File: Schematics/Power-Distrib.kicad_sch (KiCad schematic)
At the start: 49 parts, among them J102 Jack-DC, J103 Conn_01x02, J18 Jack-DC, J24 Conn_01x02, J25 Conn_01x02, J26 Screw_Terminal_01x02, J27 Conn_01x02, J28 Conn_01x02, J29 Conn_01x02, J30 Conn_01x02, J31 Conn_01x02, J32 Conn_01x02, J33 Screw_Terminal_01x02, J34 Conn_01x03, J35 Conn_01x03, J36 Conn_01x03, J37 Conn_01x03, J38 Conn_01x03, J39 Conn_01x03, J40 Conn_01x03, J41 Conn_01x03, J42 Conn_01x03, J43 Screw_Terminal_01x02, K1 Relay_SPDT, U19 LM7805, U20 LM7805, U21 LM7812, U22 LM7912

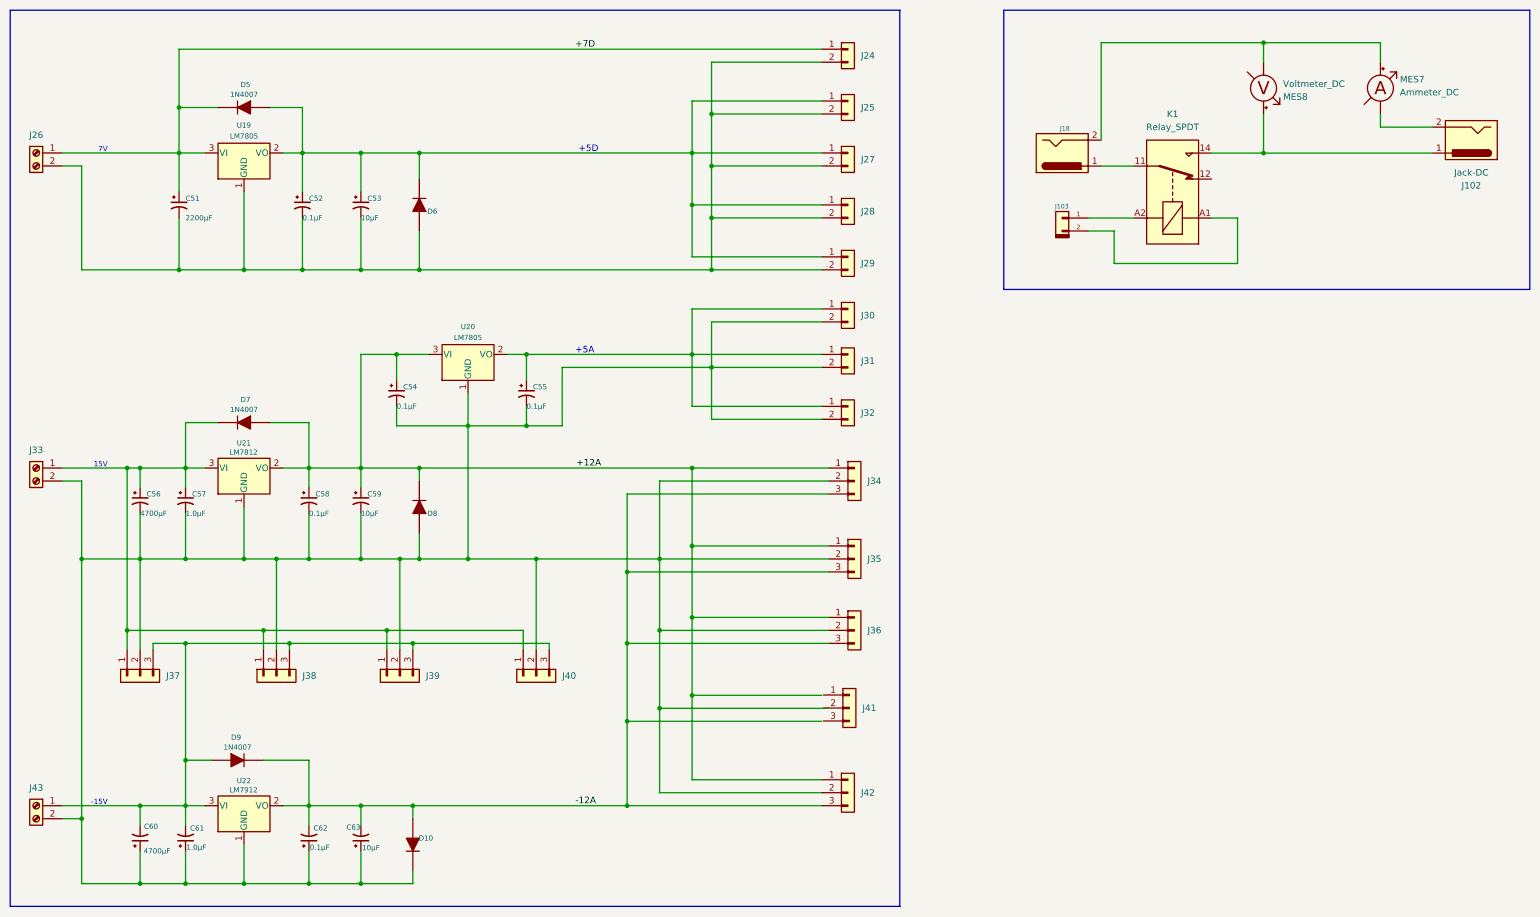
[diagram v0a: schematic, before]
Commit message: updated schematics.
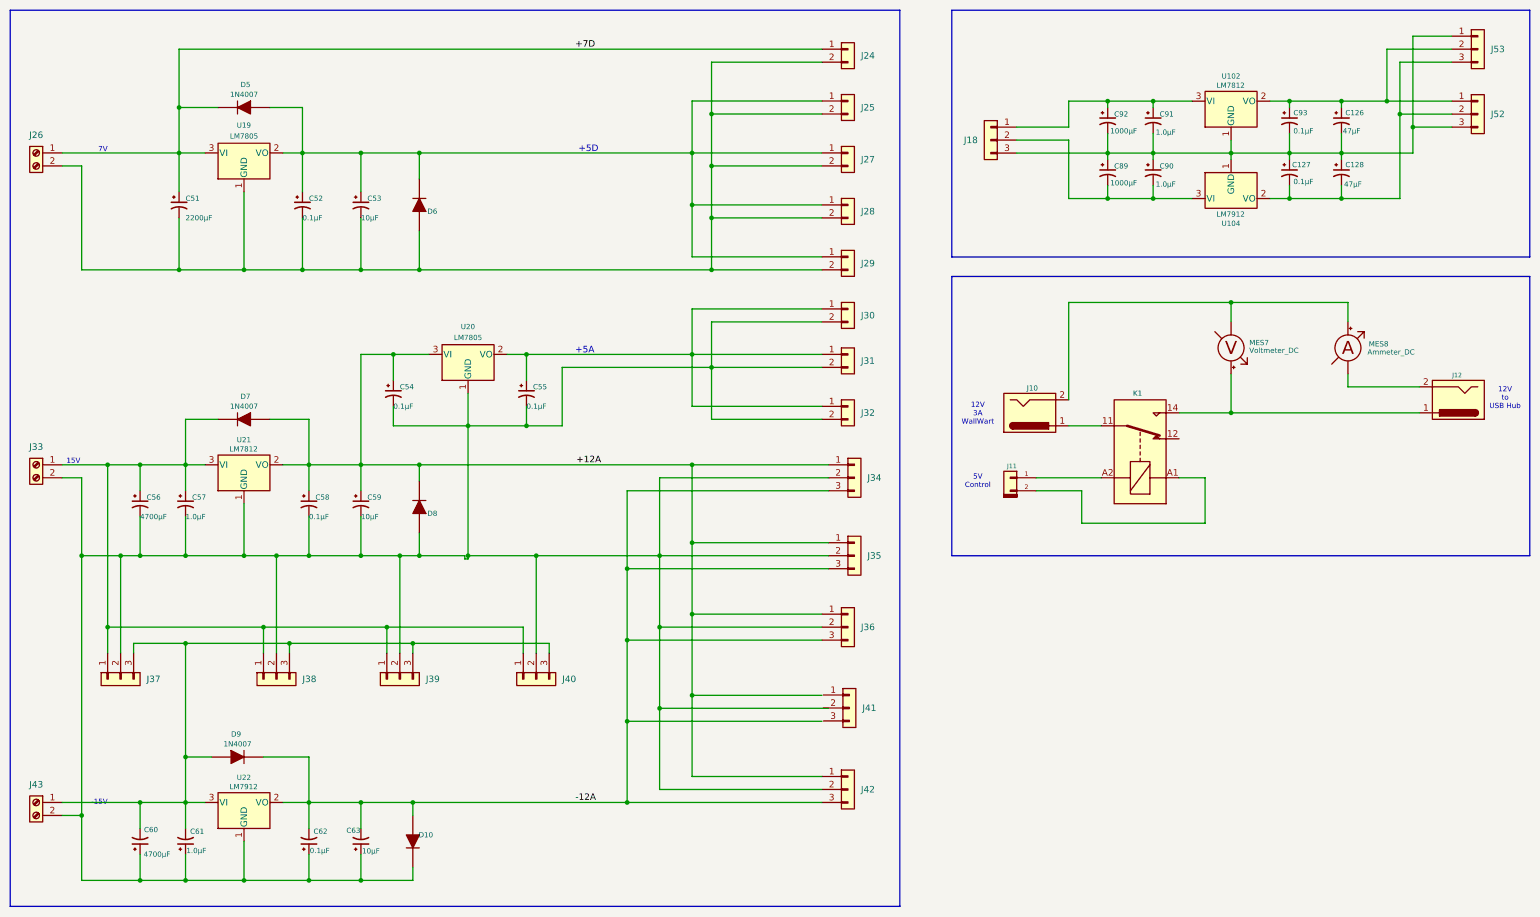
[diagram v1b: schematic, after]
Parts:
- removed J102, J18: Jack-DC, symbol Connector:Jack-DC
- removed J103: Conn_01x02, symbol My Connectors:Conn_01x02
- removed MES7: Ammeter_DC, symbol Device:Ammeter_DC
- removed MES8: Voltmeter_DC, symbol Device:Voltmeter_DC
- added C126, C128: 47µF, symbol Device:C_Polarized_Small_US
- added C127, C93: 0.1µF, symbol Device:C_Polarized_Small_US
- added C89, C92: 1000µF, symbol Device:C_Polarized_Small_US
- added C90, C91: 1.0µF, symbol Device:C_Polarized_Small_US
- added J10, J12: Jack-DC, symbol Connector:Jack-DC
- added J11: Conn_01x02, symbol My Connectors:Conn_01x02
- added J18, J52, J53: Conn_01x03, symbol Connector_Generic:Conn_01x03
- added MES7: Voltmeter_DC, symbol Device:Voltmeter_DC
- added MES8: Ammeter_DC, symbol Device:Ammeter_DC
- added U102: LM7812, symbol Regulator_Linear:LM1117-5.0
- added U104: LM7912, symbol Regulator_Linear:LM1117-5.0
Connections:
- net at K1.11: now also J10.1
- net at K1.14: now also J12.1, MES7.2 (+)
- net at K1.A2: now also J11.1 (Pin_1)
- net at K1.A1: now also J11.2 (Pin_2)
- new net: C126.2, C127.1, C128.1, C89.1, C90.1, C91.2, C92.2, C93.2, J18.3 (Pin_3), J52.3 (Pin_3), J53.1 (Pin_1), U102.1 (GND), U104.1 (GND)
- new net: C126.1, C93.1, J52.1 (Pin_1), J53.2 (Pin_2), U102.2 (VO)
- new net: C127.2, C128.2, J52.2 (Pin_2), J53.3 (Pin_3), U104.2 (VO)
- new net: C91.1, C92.1, J18.1 (Pin_1), U102.3 (VI)
- new net: C89.2, C90.2, J18.2 (Pin_2), U104.3 (VI)
- new net: J10.2, MES7.1 (-), MES8.2 (+)
- new net: J12.2, MES8.1 (-)
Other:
- note added: "12V 3A WallWart"
- note added: "12V to USB Hub"
- note added: "5V Control"
- moved on the sheet: C54, C56, C57, C58, C59, C60, C61, C62, C63, D10, D7, D9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
